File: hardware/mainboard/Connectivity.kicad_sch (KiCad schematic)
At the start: 15 parts, among them U6 MCP2542FD-E/MF, U7 MCP2542FD-E/MF

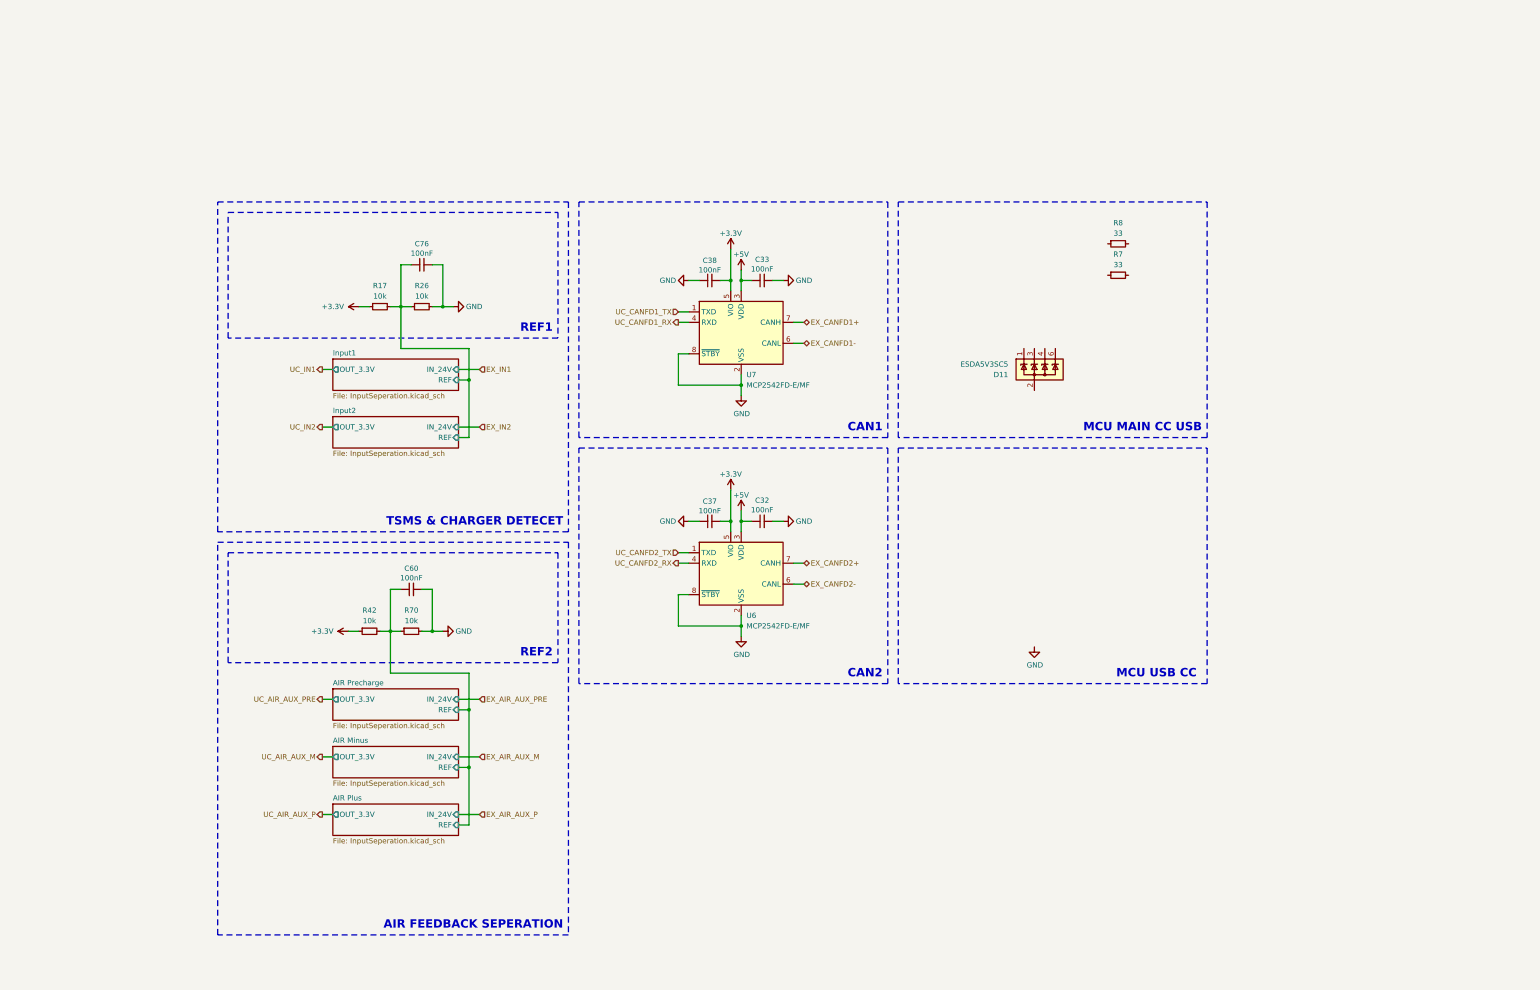
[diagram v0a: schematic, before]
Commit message: schematic?
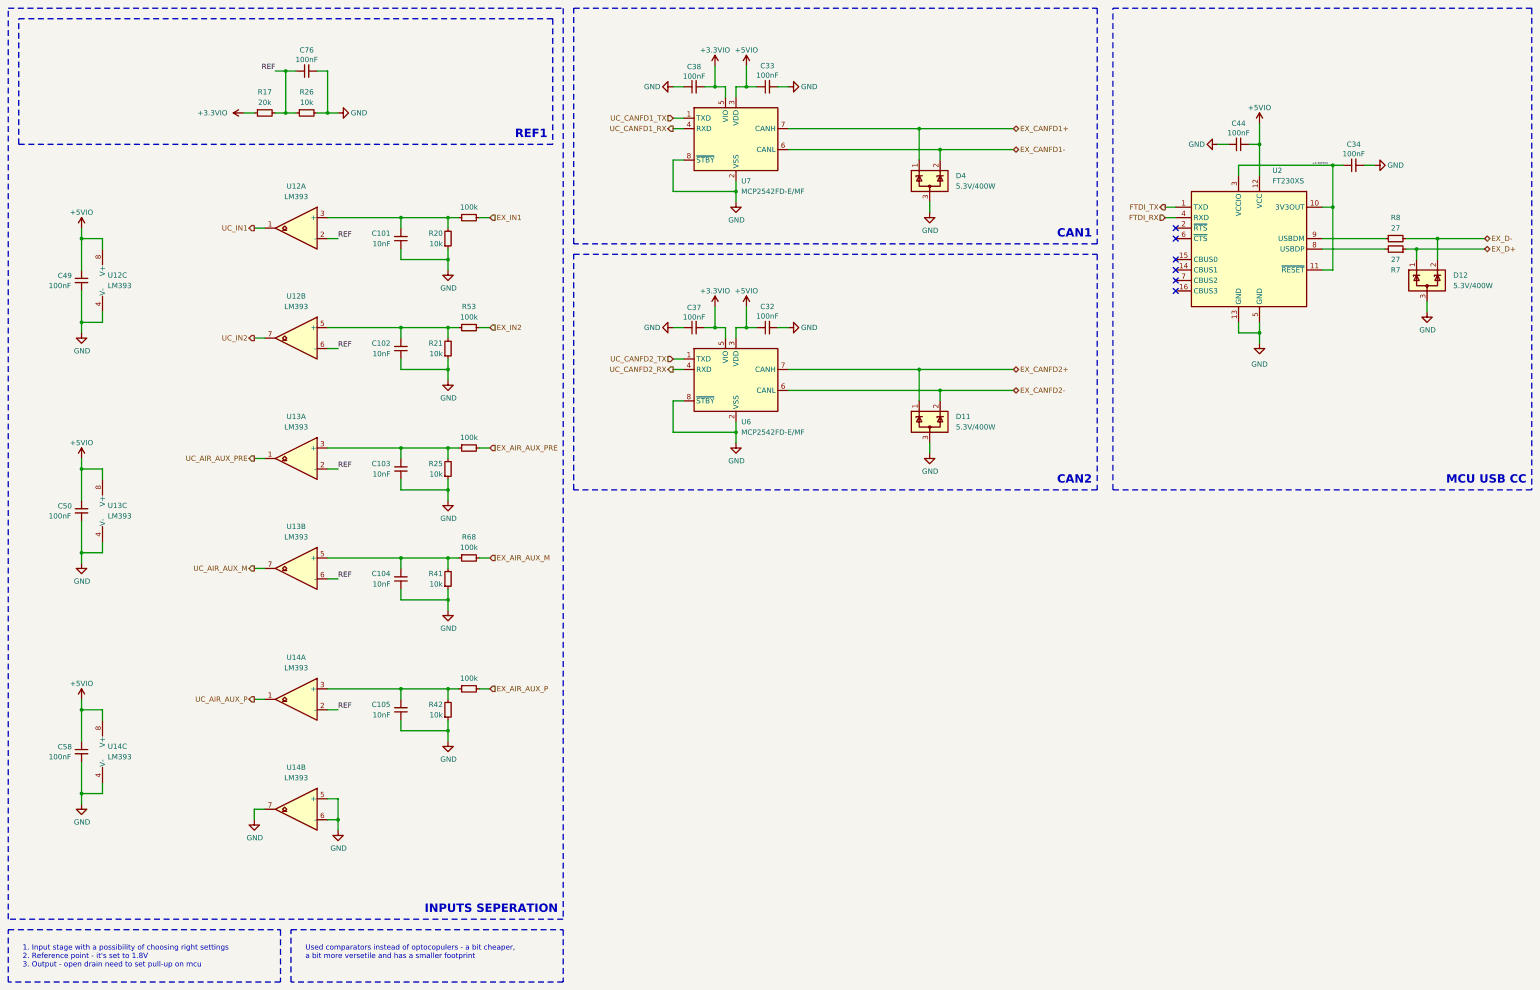
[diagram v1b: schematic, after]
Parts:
- removed C60: 100nF, Capacitor_SMD:C_0603_1608Metric, symbol Device:C_Small
- removed D11: ESDA5V3SC5, Package_TO_SOT_SMD:SOT-23-6, symbol Power_Protection:ESDA5V3SC5
- added C101, C102, C103, C104, C105: 10nF, Capacitor_SMD:C_0603_1608Metric, symbol Device:C_Small
- added C34, C44, C49, C50, C58: 100nF, Capacitor_SMD:C_0603_1608Metric, symbol Device:C_Small
- added D11, D12, D4: 5.3V/400W, Package_TO_SOT_SMD:SOT-23-3, symbol Power_Protection:ESDA5V3L
- added R20, R21, R25, R41: 10k, Resistor_SMD:R_0603_1608Metric, symbol Device:R_Small
- added R49, R53, R63, R68: 100k, Resistor_SMD:R_0603_1608Metric, symbol Device:R_Small
- added U12, U13, U14: LM393, Package_SO:VSSOP-8_3x3mm_P0.65mm, symbol Comparator:LM393
- added U2: FT230XS, Package_SO:SSOP-16_3.9x4.9mm_P0.635mm, symbol Interface_USB:FT230XS
- R17: value 10k -> 20k
- R7, R8: value 33 -> 27
- R70: value 10k -> 100k
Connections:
- net EX_AIR_AUX_M: now also R68.2
- net EX_AIR_AUX_P: now also R70.2
- net EX_AIR_AUX_PRE: now also R63.2
- net EX_CANFD1+: now also D4.1 (K)
- net EX_CANFD1-: now also D4.2 (K)
- net EX_CANFD2+: now also D11.1 (K)
- net EX_CANFD2-: now also D11.2 (K)
- net EX_IN1: now also R49.2
- net EX_IN2: now also R53.2
- net GND: now also R42.1, C101.1, C102.1, C103.1, C104.1, C105.1, C34.2, C44.2, C49.2, C50.2, C58.2, D11.3 (A), D12.3 (A), D4.3 (A), R20.1, R21.1, R25.1, R41.1, U12.4 (V-), U13.4 (V-), U14.4 (V-), U14.5 (+), U14.6 (-), U14.7, U2.13 (GND), U2.5 (GND); no longer R70.2
- net UC_AIR_AUX_M: now also U13.7
- net UC_AIR_AUX_P: now also U14.1
- net UC_AIR_AUX_PRE: now also U13.1
- net UC_IN1: now also U12.1
- net UC_IN2: now also U12.7
- net at R8.1: now also U2.9 (USBDM)
- net EX_D-: now reaches R8.2
- net EX_D-: now also D12.2 (K)
- net EX_D+: now reaches R7.1
- net EX_D+: now also D12.1 (K)
- net at R7.2: now also U2.8 (USBDP)
- net +3.3V renamed +3.3VIO
- net +3.3VIO: no longer R42.1
- net +5V renamed +5VIO
- net +5VIO: now also C44.1, C49.1, C50.1, C58.1, U12.8 (V+), U13.8 (V+), U14.8 (V+), U2.12 (VCC)
- net AIR Minus/REF: no longer names the net of R42.2, R70.1
- net AIR Minus/REF: now also C105.2, U14.3 (+)
- net Input1/REF renamed REF
- net REF: now also U12.2 (-), U12.6 (-), U13.2 (-), U13.6 (-), U14.2 (-)
- new net: C101.2, R20.2, R49.1, U12.3 (+)
- new net: C103.2, R25.2, R63.1, U13.3 (+)
- new net: C104.2, R41.2, R68.1, U13.5 (+)
- new net: C102.2, R21.2, R53.1, U12.5 (+)
- new net +3.3VFTDI: C34.1, U2.10 (3V3OUT), U2.11 (~{RESET}), U2.3 (VCCIO)
- new net FTDI_RX: U2.4 (RXD)
- new net FTDI_TX: U2.1 (TXD)
- no-connect marks 0 -> 6
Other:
- removed sheet AIR Minus
- removed sheet AIR Plus
- removed sheet AIR Precharge
- removed sheet Input1
- removed sheet Input2
- note added: "INPUTS SEPERATION"
- note removed: "AIR FEEDBACK SEPERATION"
- note removed: "MCU MAIN CC USB"
- note removed: "REF2"
- note removed: "TSMS & CHARGER DETECET"
- moved on the sheet: C32, C33, C37, C38, C76, R17, R26, R7, R8, U6, U7
